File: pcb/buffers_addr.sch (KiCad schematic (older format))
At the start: 24 parts, among them U3 74LVCH162245A, U4 74LVCH162245A

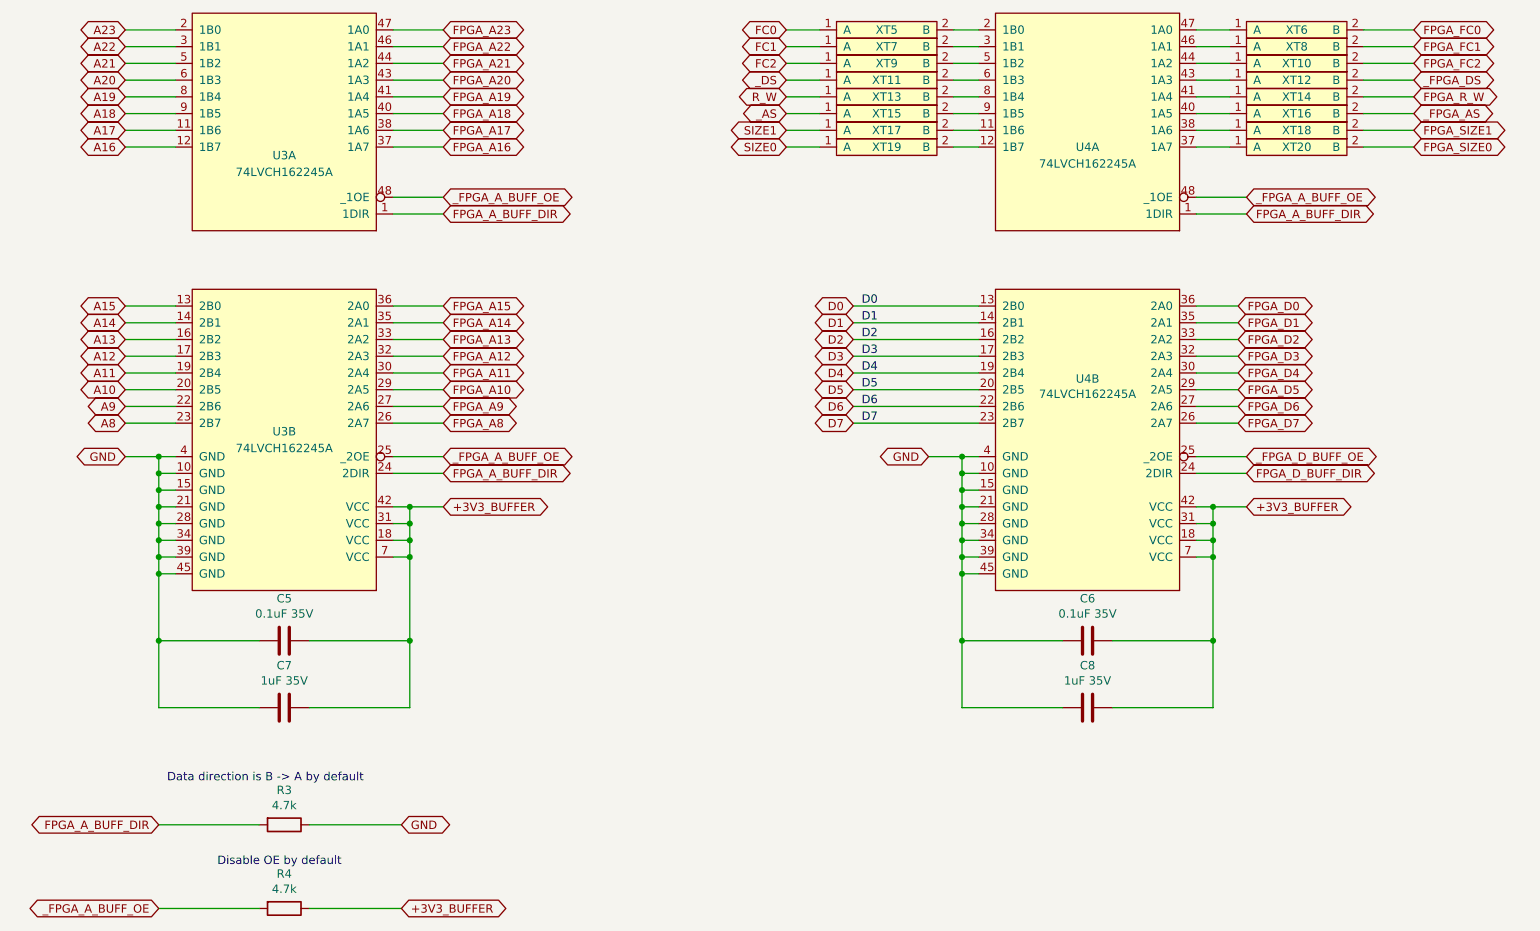
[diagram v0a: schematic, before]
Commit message: some more work done
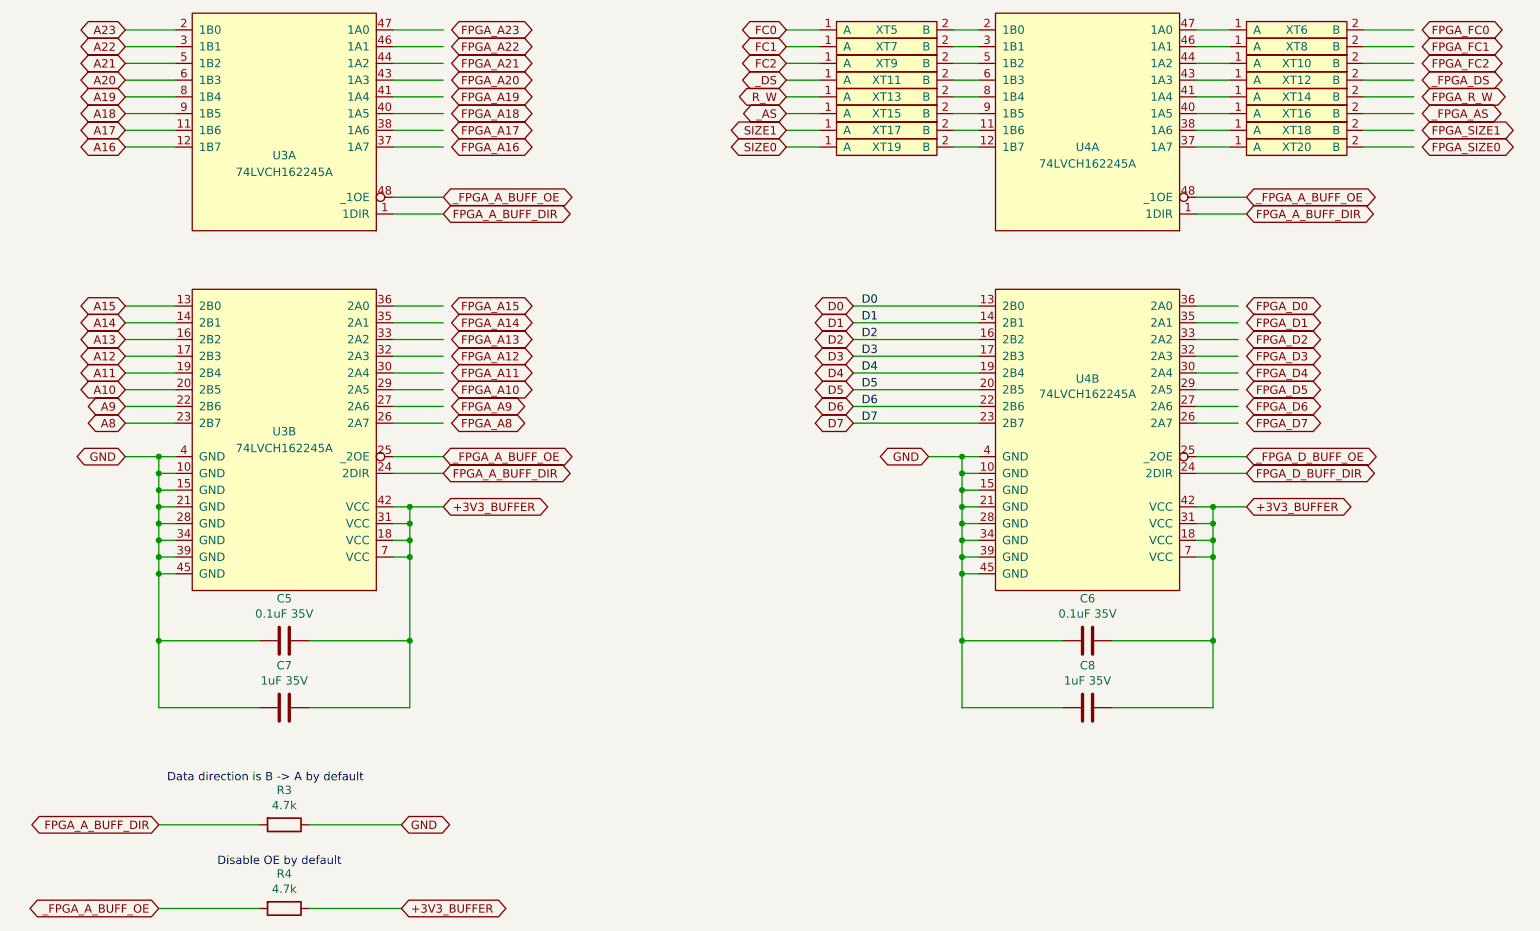
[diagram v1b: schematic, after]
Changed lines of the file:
@@
 Text GLabel 3950 6800 2    50   BiDi ~ 0
 +3V3_BUFFER
-Text GLabel 4200 1550 2    50   BiDi ~ 0
+Text GLabel 4250 1550 2    50   BiDi ~ 0
 FPGA_A23
-Text GLabel 4200 1650 2    50   BiDi ~ 0
+Text GLabel 4250 1650 2    50   BiDi ~ 0
 FPGA_A22
-Text GLabel 4200 1750 2    50   BiDi ~ 0
+Text GLabel 4250 1750 2    50   BiDi ~ 0
 FPGA_A21
-Text GLabel 4200 1850 2    50   BiDi ~ 0
+Text GLabel 4250 1850 2    50   BiDi ~ 0
 FPGA_A20
-Text GLabel 4200 1950 2    50   BiDi ~ 0
+Text GLabel 4250 1950 2    50   BiDi ~ 0
 FPGA_A19
-Text GLabel 4200 2050 2    50   BiDi ~ 0
+Text GLabel 4250 2050 2    50   BiDi ~ 0
 FPGA_A18
-Text GLabel 4200 2150 2    50   BiDi ~ 0
+Text GLabel 4250 2150 2    50   BiDi ~ 0
 FPGA_A17
-Text GLabel 4200 2250 2    50   BiDi ~ 0
+Text GLabel 4250 2250 2    50   BiDi ~ 0
 FPGA_A16
-Text GLabel 4200 3200 2    50   BiDi ~ 0
+Text GLabel 4250 3200 2    50   BiDi ~ 0
 FPGA_A15
-Text GLabel 4200 3300 2    50   BiDi ~ 0
+Text GLabel 4250 3300 2    50   BiDi ~ 0
 FPGA_A14
-Text GLabel 4200 3400 2    50   BiDi ~ 0
+Text GLabel 4250 3400 2    50   BiDi ~ 0
 FPGA_A13
-Text GLabel 4200 3500 2    50   BiDi ~ 0
+Text GLabel 4250 3500 2    50   BiDi ~ 0
 FPGA_A12
-Text GLabel 4200 3600 2    50   BiDi ~ 0
+Text GLabel 4250 3600 2    50   BiDi ~ 0
 FPGA_A11
-Text GLabel 4200 3700 2    50   BiDi ~ 0
+Text GLabel 4250 3700 2    50   BiDi ~ 0
 FPGA_A10
-Text GLabel 4200 3800 2    50   BiDi ~ 0
+Text GLabel 4250 3800 2    50   BiDi ~ 0
 FPGA_A9
-Text GLabel 4200 3900 2    50   BiDi ~ 0
+Text GLabel 4250 3900 2    50   BiDi ~ 0
 FPGA_A8
-Text GLabel 10000 2050 2    50   BiDi ~ 0
+Text GLabel 10050 2050 2    50   BiDi ~ 0
 _FPGA_AS
-Text GLabel 10000 1850 2    50   BiDi ~ 0
+Text GLabel 10050 1850 2    50   BiDi ~ 0
 _FPGA_DS
-Text GLabel 10000 1950 2    50   BiDi ~ 0
+Text GLabel 10050 1950 2    50   BiDi ~ 0
 FPGA_R_W
-Text GLabel 10000 2250 2    50   BiDi ~ 0
+Text GLabel 10050 2250 2    50   BiDi ~ 0
 FPGA_SIZE0
-Text GLabel 10000 2150 2    50   BiDi ~ 0
+Text GLabel 10050 2150 2    50   BiDi ~ 0
 FPGA_SIZE1
-Text GLabel 10000 1750 2    50   BiDi ~ 0
+Text GLabel 10050 1750 2    50   BiDi ~ 0
 FPGA_FC2
-Text GLabel 10000 1650 2    50   BiDi ~ 0
+Text GLabel 10050 1650 2    50   BiDi ~ 0
 FPGA_FC1
-Text GLabel 10000 1550 2    50   BiDi ~ 0
+Text GLabel 10050 1550 2    50   BiDi ~ 0
 FPGA_FC0
 Wire Wire Line
@@
 Text GLabel 6650 3200 0    50   BiDi ~ 0
 D0
-Text GLabel 8950 3900 2    50   BiDi ~ 0
+Text GLabel 9000 3900 2    50   BiDi ~ 0
 FPGA_D7
-Text GLabel 8950 3800 2    50   BiDi ~ 0
+Text GLabel 9000 3800 2    50   BiDi ~ 0
 FPGA_D6
-Text GLabel 8950 3700 2    50   BiDi ~ 0
+Text GLabel 9000 3700 2    50   BiDi ~ 0
 FPGA_D5
-Text GLabel 8950 3600 2    50   BiDi ~ 0
+Text GLabel 9000 3600 2    50   BiDi ~ 0
 FPGA_D4
-Text GLabel 8950 3500 2    50   BiDi ~ 0
+Text GLabel 9000 3500 2    50   BiDi ~ 0
 FPGA_D3
-Text GLabel 8950 3400 2    50   BiDi ~ 0
+Text GLabel 9000 3400 2    50   BiDi ~ 0
 FPGA_D2
-Text GLabel 8950 3300 2    50   BiDi ~ 0
+Text GLabel 9000 3300 2    50   BiDi ~ 0
 FPGA_D1
-Text GLabel 8950 3200 2    50   BiDi ~ 0
+Text GLabel 9000 3200 2    50   BiDi ~ 0
 FPGA_D0
 Text GLabel 6650 3900 0    50   BiDi ~ 0
